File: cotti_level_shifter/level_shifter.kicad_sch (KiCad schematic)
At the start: 6 parts, among them U1 74LVC1T45DW-7

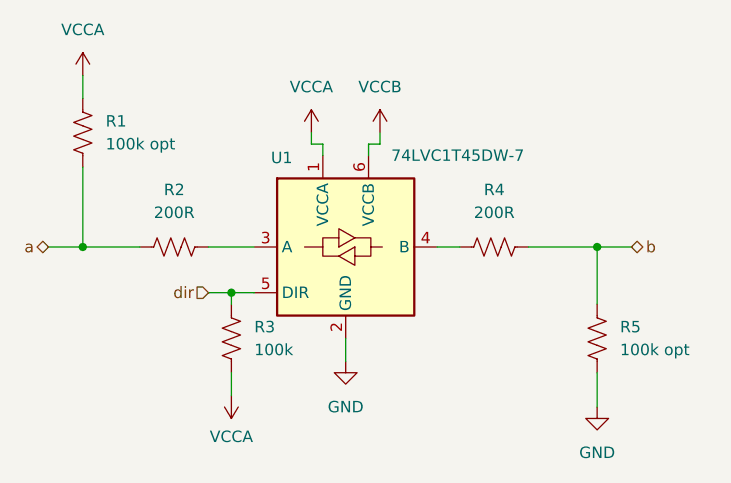
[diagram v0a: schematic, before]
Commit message: feat: level shifter gerbers
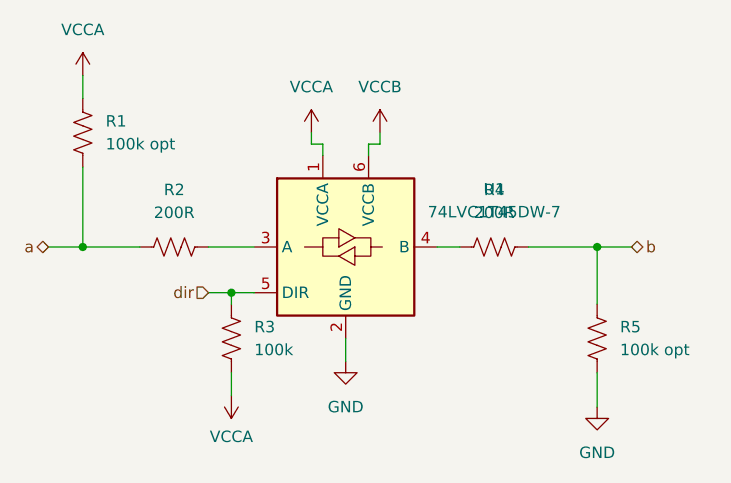
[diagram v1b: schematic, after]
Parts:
- removed U1: 74LVC1T45DW-7, Package_TO_SOT_SMD:SOT-363_SC-70-6, symbol Logic_LevelTranslator:SN74LVC1T45DCK
- added U1: 74LVC1T45DW-7, Package_TO_SOT_SMD:SOT-363_SC-70-6, symbol cotti_ic:voltage_level_translator
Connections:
- net GND: now also U1.2 (GND)
- net VCCA: now also U1.1 (VCCA)
- net VCCB: now also U1.6 (VCCB)
- net dir: now also U1.5 (DIR)
- net at R2.2: now also U1.3 (A)
- net at R4.1: now also U1.4 (B)
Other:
- company: (none) -> Cotti
- title: (none) -> Level Shifter Module
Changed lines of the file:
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@@
 	(generator_version "9.0")
 	(paper "A4")
+	(title_block
+		(title "Level Shifter Module")
+		(date "2026-01-17")
+		(rev "0.0")
+		(company "Cotti")
+	)
 	(junction
 		(at 115.57 86.36)
@@
 	)
 	(symbol
-		(lib_id "Logic_LevelTranslator:SN74LVC1T45DCK")
-		(at 144.78 86.36 0)
-		(unit 1)
-		(exclude_from_sim no)
-		(in_bom yes)
-		(on_board yes)
-		(dnp no)
-		(property "Reference" "U1"
-			(at 137.668 76.454 0)
-			(effects
-				(font
-					(size 1.27 1.27)
-				)
-			)
-		)
-		(property "Value" "74LVC1T45DW-7"
-			(at 157.226 76.2 0)
-			(effects
-				(font
-					(size 1.27 1.27)
-				)
-			)
-		)
-		(property "Footprint" "Package_TO_SOT_SMD:SOT-363_SC-70-6"
-			(at 144.78 97.79 0)
-			(effects
-				(font
-					(size 1.27 1.27)
-				)
-				(hide yes)
-			)
-		)
-		(property "Datasheet" "http://www.ti.com/lit/ds/symlink/sn74lvc1t45.pdf"
-			(at 121.92 102.87 0)
-			(effects
-				(font
-					(size 1.27 1.27)
-				)
-				(hide yes)
-			)
-		)
-		(property "Description" "Single-Bit Dual-Supply Bus Transceiver With Configurable Voltage Translation and 3-State Outputs, SOT-363"
-			(at 144.78 86.36 0)
-			(effects
-				(font
-					(size 1.27 1.27)
-				)
-				(hide yes)
-			)
-		)
-		(property "Digikey" "https://www.digikey.com/en/products/detail/diodes-incorporated/74LVC1T45DW-7/5427266"
-			(at 144.78 86.36 0)
-			(effects
-				(font
-					(size 1.27 1.27)
-				)
-				(hide yes)
-			)
-		)
-		(property "Digikey P/N" "31-74LVC1T45DW-7CT-ND"
-			(at 144.78 86.36 0)
-			(effects
-				(font
-					(size 1.27 1.27)
-				)
-				(hide yes)
-			)
-		)
-		(property "Mfr." "Diodes Incorporated"
-			(at 144.78 86.36 0)
-			(effects
-				(font
-					(size 1.27 1.27)
-				)
-				(hide yes)
-			)
-		)
-		(property "Mfr. P/N" "74LVC1T45DW-7"
-			(at 144.78 86.36 0)
-			(effects
-				(font
-					(size 1.27 1.27)
-				)
-				(hide yes)
-			)
-		)
-		(pin "5"
-		)
-		(pin "1"
-		)
-		(pin "2"
-		)
-		(pin "6"
-		)
-		(pin "4"
-		)
-		(pin "3"
-		)
-		(instances
-			(project "cotti_level_shifter"
-				(path "/9157c1e3-b0d9-40ec-a93b-dbe68aa8cbb2/01aab807-bbb4-4afa-aa40-b9e9d43e83d4"
-					(reference "U1")
-					(unit 1)
-				)
-				(path "/9157c1e3-b0d9-40ec-a93b-dbe68aa8cbb2/30f197c9-0cd8-437a-a5b7-774f1b2516e0"
-					(reference "U3")
-					(unit 1)
-				)
-				(path "/9157c1e3-b0d9-40ec-a93b-dbe68aa8cbb2/4c84f02b-2522-49cd-b2e7-e24a49a97dac"
-					(reference "U8")
-					(unit 1)
-				)
-				(path "/9157c1e3-b0d9-40ec-a93b-dbe68aa8cbb2/63f08a8f-7e54-4a04-8424-a7a423b9d454"
-					(reference "U2")
-					(unit 1)
-				)
-				(path "/9157c1e3-b0d9-40ec-a93b-dbe68aa8cbb2/974f5a64-b060-4b01-8908-45bb104fb08e"
-					(reference "U7")
-					(unit 1)
-				)
-				(path "/9157c1e3-b0d9-40ec-a93b-dbe68aa8cbb2/9f67e98d-9a78-4046-8f19-e539622706a5"
-					(reference "U6")
-					(unit 1)
-				)
-				(path "/9157c1e3-b0d9-40ec-a93b-dbe68aa8cbb2/a2268e70-50b9-4576-8fc4-fe7046032005"
-					(reference "U4")
-					(unit 1)
-				)
-				(path "/9157c1e3-b0d9-40ec-a93b-dbe68aa8cbb2/ec8e5640-8d6c-4b64-928d-01aae8347ab5"
-					(reference "U5")
-					(unit 1)
-				)
-			)
-		)
-	)
-	(symbol
 		(lib_id "Device:R_US")
 		(at 161.29 86.36 90)
@@
 					(unit 1)
 				)
+			)
+		)
+	)
+	(symbol
+		(lib_id "cotti_ic:voltage_level_translator")
+		(at 144.78 86.36 0)
+		(unit 1)
+		(exclude_from_sim no)
+		(in_bom yes)
+		(on_board yes)
+		(dnp no)
+		(fields_autoplaced yes)
+		(property "Reference" "U1"
+			(at 161.29 79.9398 0)
+			(effects
+				(font
+					(size 1.27 1.27)
+				)
+			)
+		)
+		(property "Value" "74LVC1T45DW-7"
+			(at 161.29 82.4798 0)
+			(effects
+				(font
+					(size 1.27 1.27)
+				)
+			)
+		)
+		(property "Footprint" "Package_TO_SOT_SMD:SOT-363_SC-70-6"
+			(at 144.526 53.086 0)
+			(effects
+				(font
+					(size 1.27 1.27)
+				)
+				(hide yes)
+			)
+		)
+		(property "Datasheet" "https://www.diodes.com/assets/Datasheets/74LVC1T45.pdf"
+			(at 139.192 58.674 0)
+			(effects
+				(font
+					(size 1.27 1.27)
+				)
+				(hide yes)
+			)
+		)
+		(property "Description" "Voltage Level Translator Bidirectional 1 Circuit 1 Channel SOT-363"
+			(at 145.542 46.99 0)
+			(effects
+				(font
+					(size 1.27 1.27)
+				)
+				(hide yes)
+			)
+		)
+		(property "Digikey" "https://www.digikey.com/en/products/detail/diodes-incorporated/74LVC1T45DW-7/5427266"
+			(at 150.876 43.688 0)
+			(effects
+				(font
+					(size 1.27 1.27)
+				)
+				(hide yes)
+			)
+		)
+		(property "Mfr." "Diodes Incorporated"
+			(at 143.256 40.386 0)
+			(effects
+				(font
+					(size 1.27 1.27)
+				)
+				(hide yes)
+			)
+		)
+		(property "Mfr. P/N" "74LVC1T45DW-7"
+			(at 144.526 37.592 0)
+			(effects
+				(font
+					(size 1.27 1.27)
+				)
+				(hide yes)
+			)
+		)
+		(pin "4"
+		)
+		(pin "5"
+		)
+		(pin "1"
+		)
+		(pin "2"
+		)
+		(pin "6"
+		)
+		(pin "3"
+		)
+		(instances
+			(project ""
+				(path "/9157c1e3-b0d9-40ec-a93b-dbe68aa8cbb2/01aab807-bbb4-4afa-aa40-b9e9d43e83d4"
+					(reference "U1")
+					(unit 1)
+				)
+				(path "/9157c1e3-b0d9-40ec-a93b-dbe68aa8cbb2/30f197c9-0cd8-437a-a5b7-774f1b2516e0"
+					(reference "U3")
+					(unit 1)
+				)
+				(path "/9157c1e3-b0d9-40ec-a93b-dbe68aa8cbb2/4c84f02b-2522-49cd-b2e7-e24a49a97dac"
+					(reference "U8")
+					(unit 1)
+				)
+				(path "/9157c1e3-b0d9-40ec-a93b-dbe68aa8cbb2/63f08a8f-7e54-4a04-8424-a7a423b9d454"
+					(reference "U2")
+					(unit 1)
+				)
+				(path "/9157c1e3-b0d9-40ec-a93b-dbe68aa8cbb2/974f5a64-b060-4b01-8908-45bb104fb08e"
+					(reference "U7")
+					(unit 1)
+				)
+				(path "/9157c1e3-b0d9-40ec-a93b-dbe68aa8cbb2/9f67e98d-9a78-4046-8f19-e539622706a5"
+					(reference "U6")
+					(unit 1)
+				)
+				(path "/9157c1e3-b0d9-40ec-a93b-dbe68aa8cbb2/a2268e70-50b9-4576-8fc4-fe7046032005"
+					(reference "U4")
+					(unit 1)
+				)
+				(path "/9157c1e3-b0d9-40ec-a93b-dbe68aa8cbb2/ec8e5640-8d6c-4b64-928d-01aae8347ab5"
+					(reference "U5")
+					(unit 1)
+				)
